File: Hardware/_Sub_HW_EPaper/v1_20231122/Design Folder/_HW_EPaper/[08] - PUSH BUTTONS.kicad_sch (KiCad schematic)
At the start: 6 parts, among them SW801 SPST-NO, SW802 SPST-NO

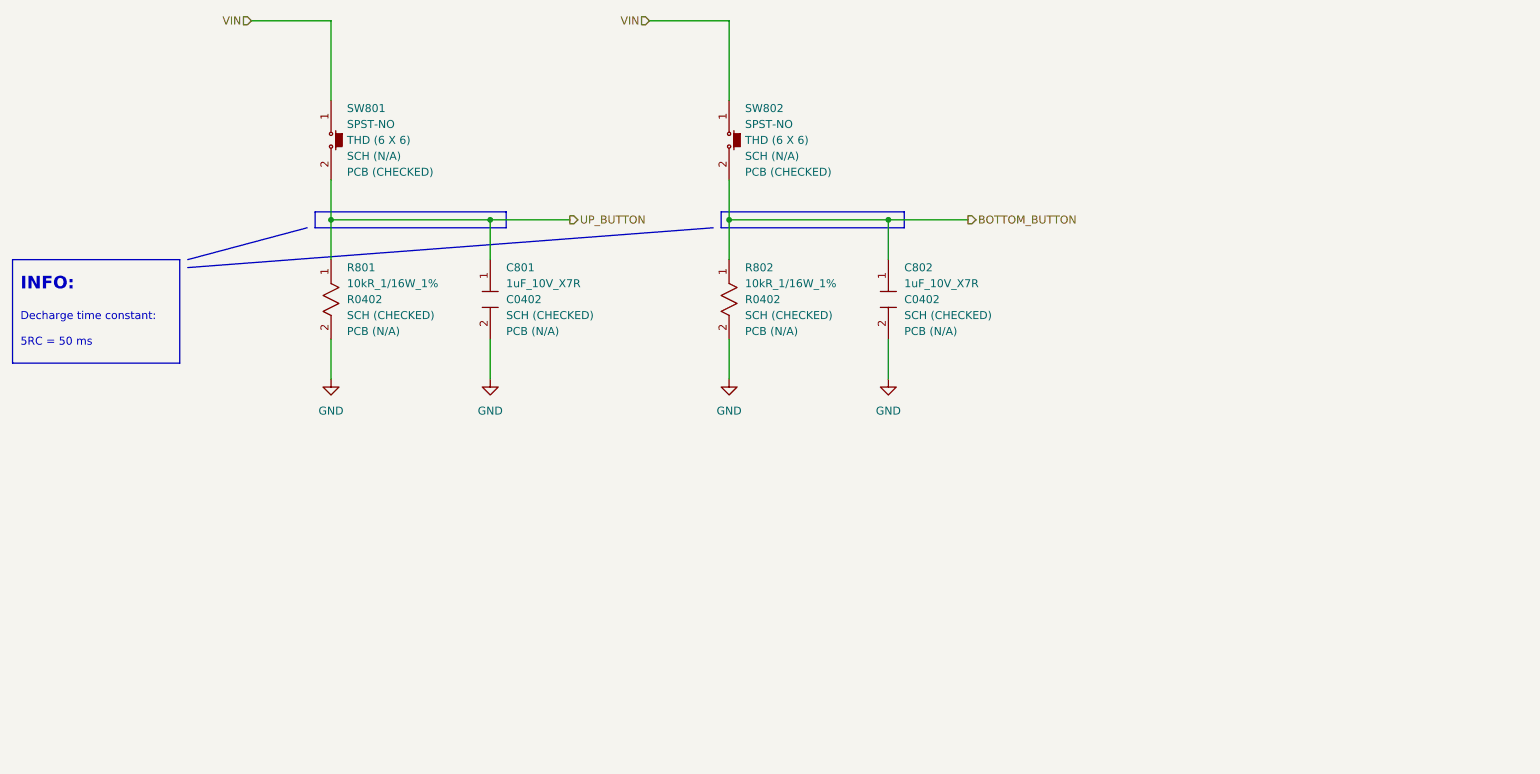
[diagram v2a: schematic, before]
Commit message: Updating file templates and structures...
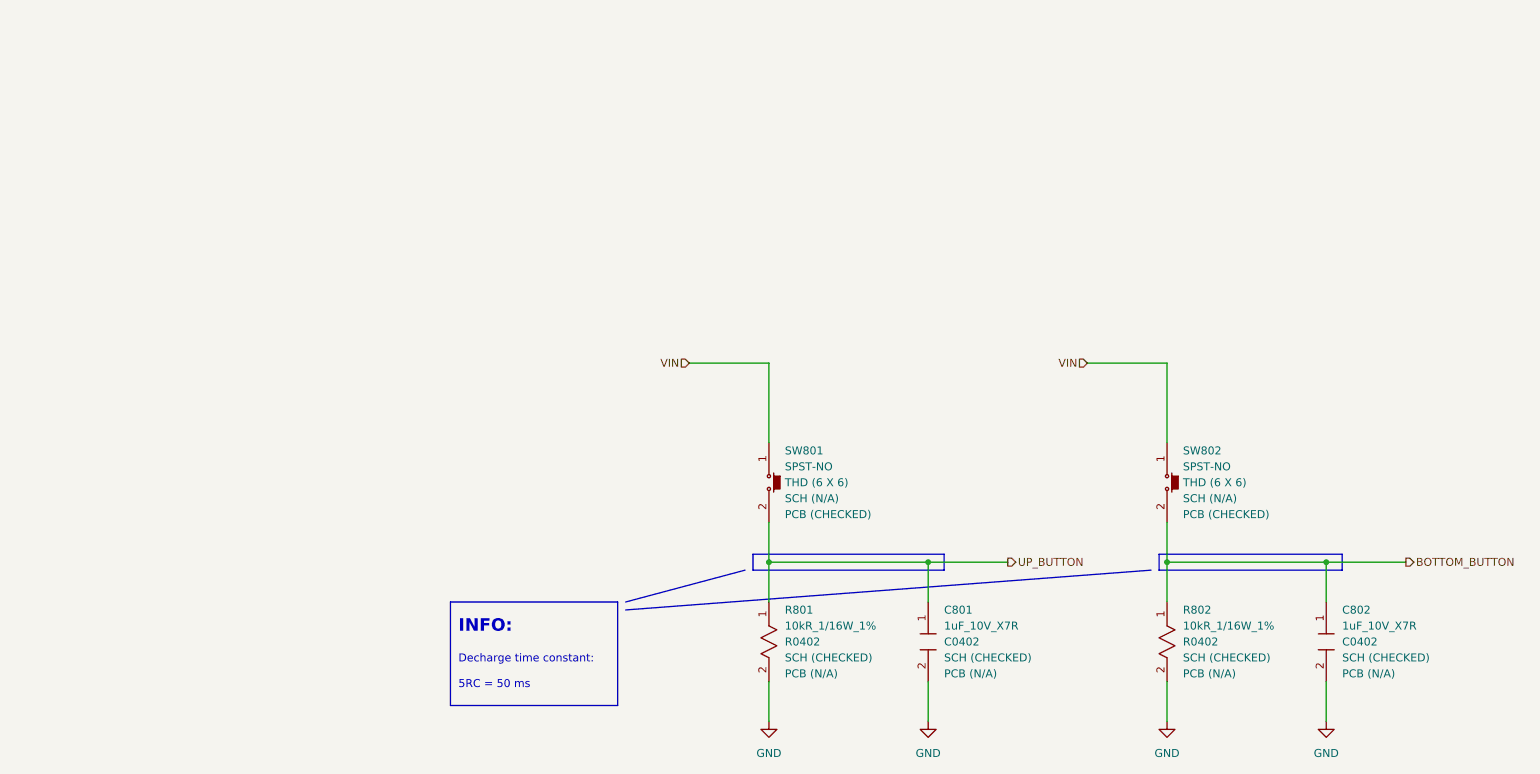
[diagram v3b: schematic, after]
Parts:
- C801, C802: Manufacturer (none) -> Murata Electronics; Part Number GRM155Z71A105KE01D -> (none); Part Number (Manufacturer) (none) -> GRM155Z71A105KE01D; Part Number (Vendor) (none) -> 490-GRM155Z71A105KE01DTR-ND; Vendor (none) -> Digikey
- R801, R802: Manufacturer (none) -> Bourns Inc.; Part Number CR0402-FX-1002GLF -> (none); Part Number (Manufacturer) (none) -> CR0402-FX-1002GLF; Part Number (Vendor) (none) -> CR0402-FX-1002GLFTR-ND; Vendor (none) -> Digikey
- SW801, SW802: Manufacturer (none) -> C&K; Part Number PTS645VH31-2 LFS -> (none); Part Number (Manufacturer) (none) -> PTS645VH31-2 LFS; Part Number (Vendor) (none) -> CKN9118-ND; Vendor (none) -> Digikey
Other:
- moved on the sheet: C801, C802, R801, R802, SW801, SW802
